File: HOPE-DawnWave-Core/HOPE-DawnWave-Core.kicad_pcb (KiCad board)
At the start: 2 copper layers, 51.8 x 51.1 mm, 50 parts, among them J1 USB_C_Receptacle_USB2.0_16P, J2 Screw_Terminal_01x02, SW1 RST, SW2 BOOT, U1 TLV62569DRL, U2 USBLC6-2P6, U3 ESP32-C6-WROOM-1, U4 MAX98357A, U5 BME688, X1 EYE_SPI_DISPLAY_FLIP

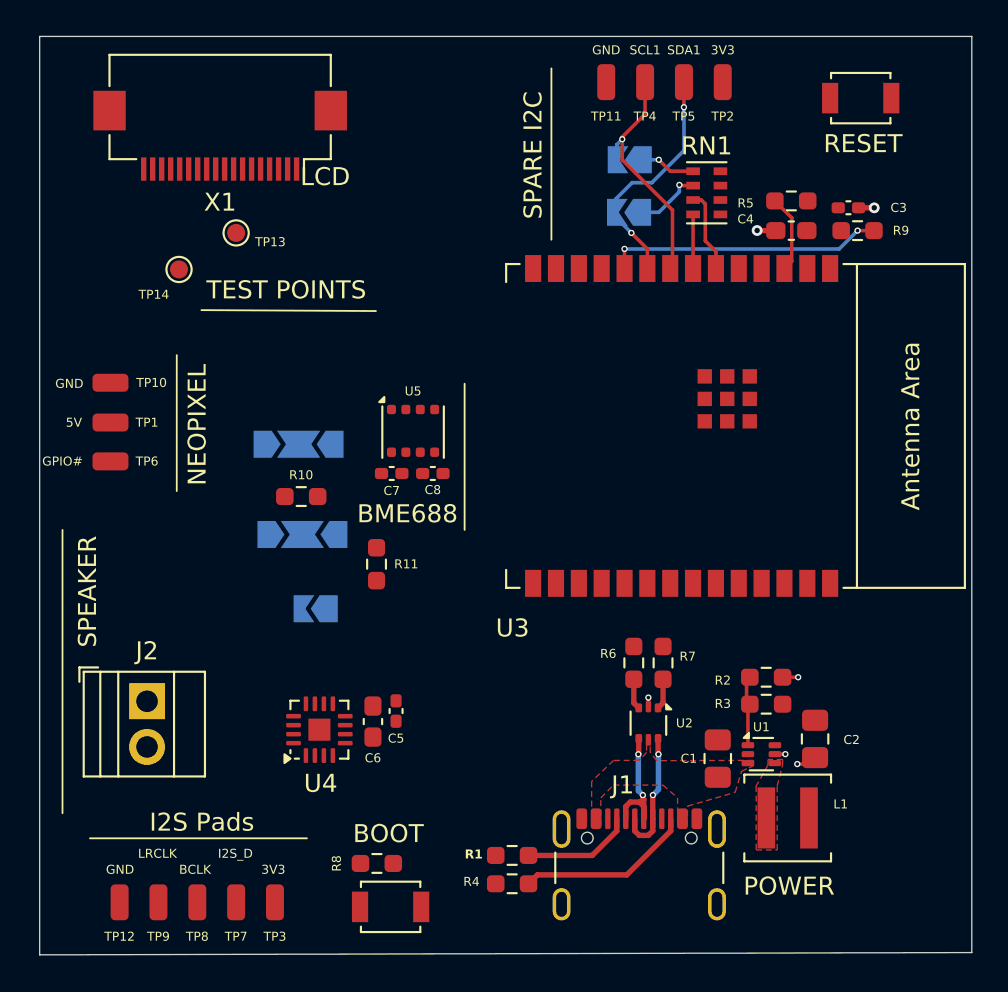
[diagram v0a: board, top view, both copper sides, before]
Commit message: big progress oops
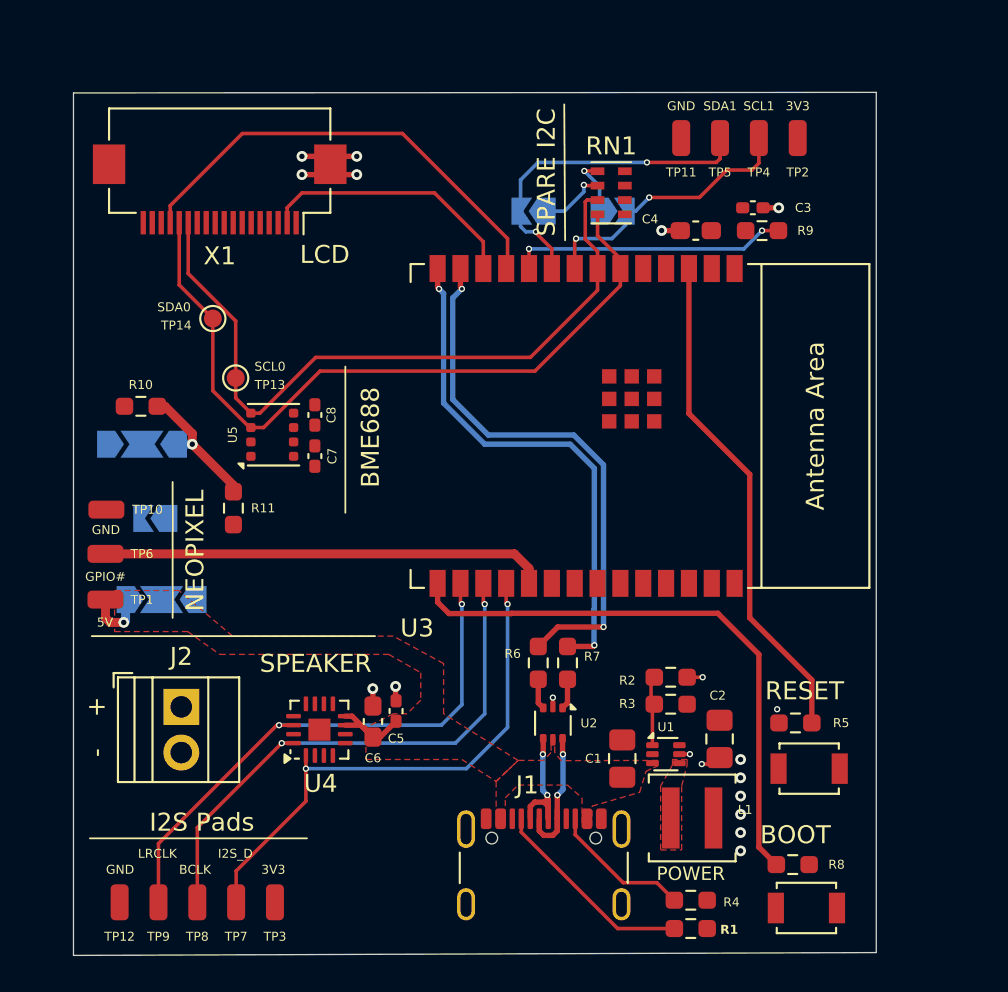
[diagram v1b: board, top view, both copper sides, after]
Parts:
- moved SW1 37.4 mm to (165.9, 107.4)
- moved R5 29.0 mm to (165.1, 104.9), turned to 0 degrees
- moved R8 23.1 mm to (164.9, 112.8)
- moved SW2 23.1 mm to (165.7, 115.2)
- moved JP4 11.5 mm to (129.9, 98.0)
- moved R1 10.7 mm to (159.3, 116.3), turned to 0 degrees
- moved JP5 10.2 mm to (129.5, 93.5)
- moved JP3 10.2 mm to (128.8, 89.4)
- moved R10 10.2 mm to (128.7, 87.3)
- moved R4 9.97 mm to (159.3, 114.8), turned to 0 degrees
- moved TP1 9.85 mm to (126.7, 98.0)
- moved R11 8.54 mm to (133.9, 93.0)
- moved TP13 8.06 mm to (134.0, 85.7)
- moved U5 7.83 mm to (136.0, 88.9), turned to 90 degrees
- moved C8 7.32 mm to (138.4, 87.8), turned to 90 degrees
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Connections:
- U3 pad 11: MCU_DRST -> MCU_TD
- U3 pad 12: MCU_TD -> MCU_BACKLIGHT
- U3 pad 16: MCU_MISO -> MCU_LRCLK
- U3 pad 17: MCU_SCLK -> MCU_BCLK
- U3 pad 18: MCU_MOSI -> MCU_I2S_D
- U3 pad 19: MCU_D/C -> GPIO_NP
- U3 pad 23: MCU_BACKLIGHT -> MCU_DRST
- U3 pad 24: MCU_LRCLK -> MCU_MISO
- U3 pad 25: MCU_BCLK -> MCU_SCLK
- U3 pad 26: MCU_I2S_D -> MCU_MOSI
- U3 pad 27: GPIO_NP -> MCU_D/C
- U3 pad 6: MCU_SCL0 -> MCU_SDA0
- U3 pad 7: MCU_SDA0 -> MCU_SCL0
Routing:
- net MCU_SDA0: track 3.01 -> 41.4 mm
- net MCU_SCL0: track 4.60 -> 40.1 mm
- net /MCU_BOOT: track 0.00 -> 32.2 mm
- net MCU_LRCLK: track 0.00 -> 30.9 mm, vias 0 -> 2
- net MCU_BCLK: track 0.00 -> 30.7 mm, vias 0 -> 2
- net /MCU_USB_D-: track 0.00 -> 30.5 mm, vias 0 -> 2
- net MCU_I2S_D: track 0.00 -> 30.0 mm, vias 0 -> 2
- net /MCU_USB_D+: track 0.00 -> 28.9 mm, vias 0 -> 2
- net MCU_TD: track 0.00 -> 25.5 mm
- net GPIO_NP: track 0.00 -> 24.7 mm
- net /MCU_EN: track 4.32 -> 28.1 mm
- net MCU_BACKLIGHT: track 0.00 -> 14.7 mm
- net VBUS: track 0.58 -> 9.51 mm, vias 1 -> 2
- net GND: track 2.41 -> 11.1 mm, vias 3 -> 9
- net +3.3V: track 2.01 -> 9.55 mm, vias 2 -> 10
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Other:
- board size 51.8 x 51.1 mm -> 44.6 x 48 mm
- board text added: "+"
- board text added: "-"
- board text added: "SCL0"
- board text added: "SCL1_PU"
- board text added: "SDA0"
- board text added: "SDA1_PU"
- board text removed: "TEST POINTS"
